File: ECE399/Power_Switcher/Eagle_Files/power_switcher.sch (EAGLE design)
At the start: 69 parts, among them J1 BANNANA_DEV, J2 BANNANA_DEV, J3 BANNANA_DEV, J4 BANNANA_DEV, J5 BANNANA_DEV, J6 BANNANA_DEV, J7 BANNANA_DEV, Q1 TRANSISTOR_DEV, Q2 TRANSISTOR_DEV, Q3 TRANSISTOR_DEV, Q4 TRANSISTOR_DEV, U1 DC_DC_DEV, U2 DC_DC_DEV, U3 GATE_DRIVER_DEV, U4 GATE_DRIVER_DEV, U5 PWM_DRIVER_DEV

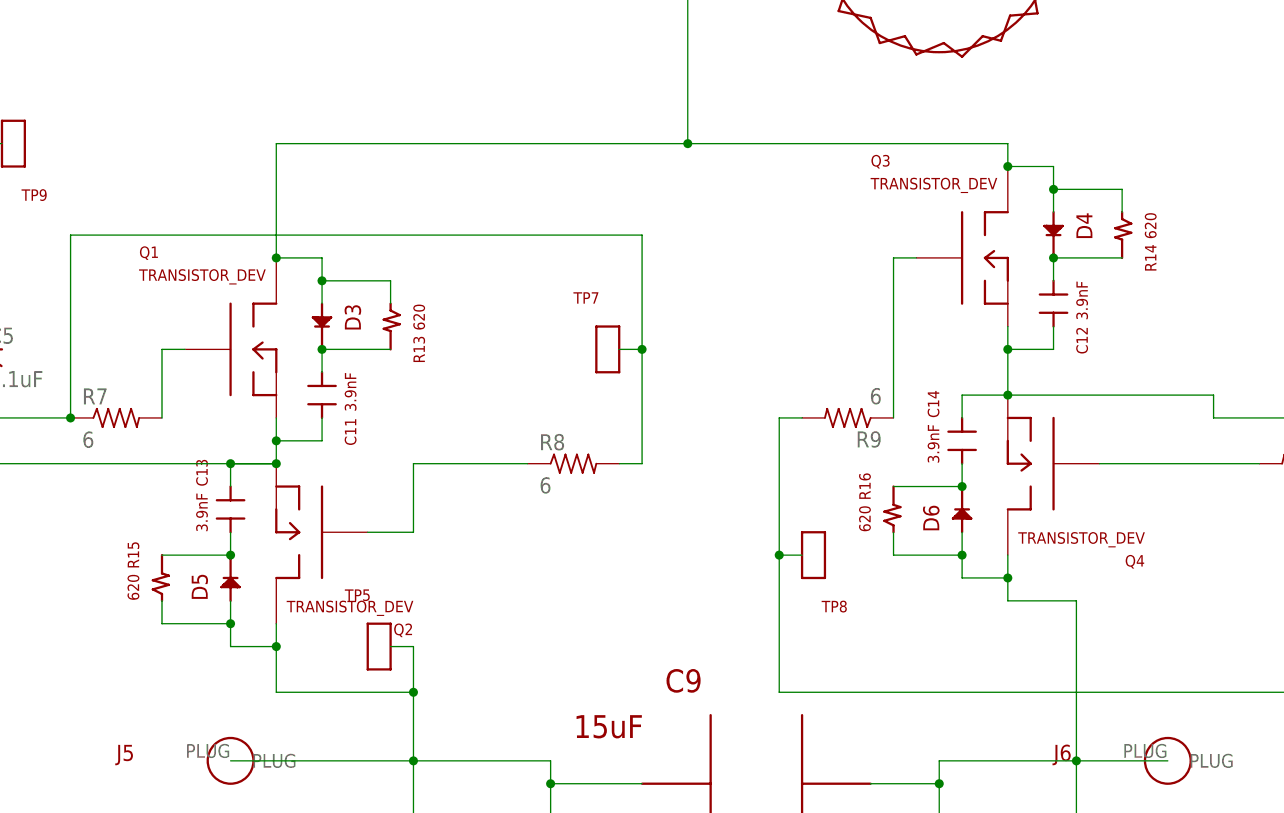
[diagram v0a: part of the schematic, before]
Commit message: right diode added
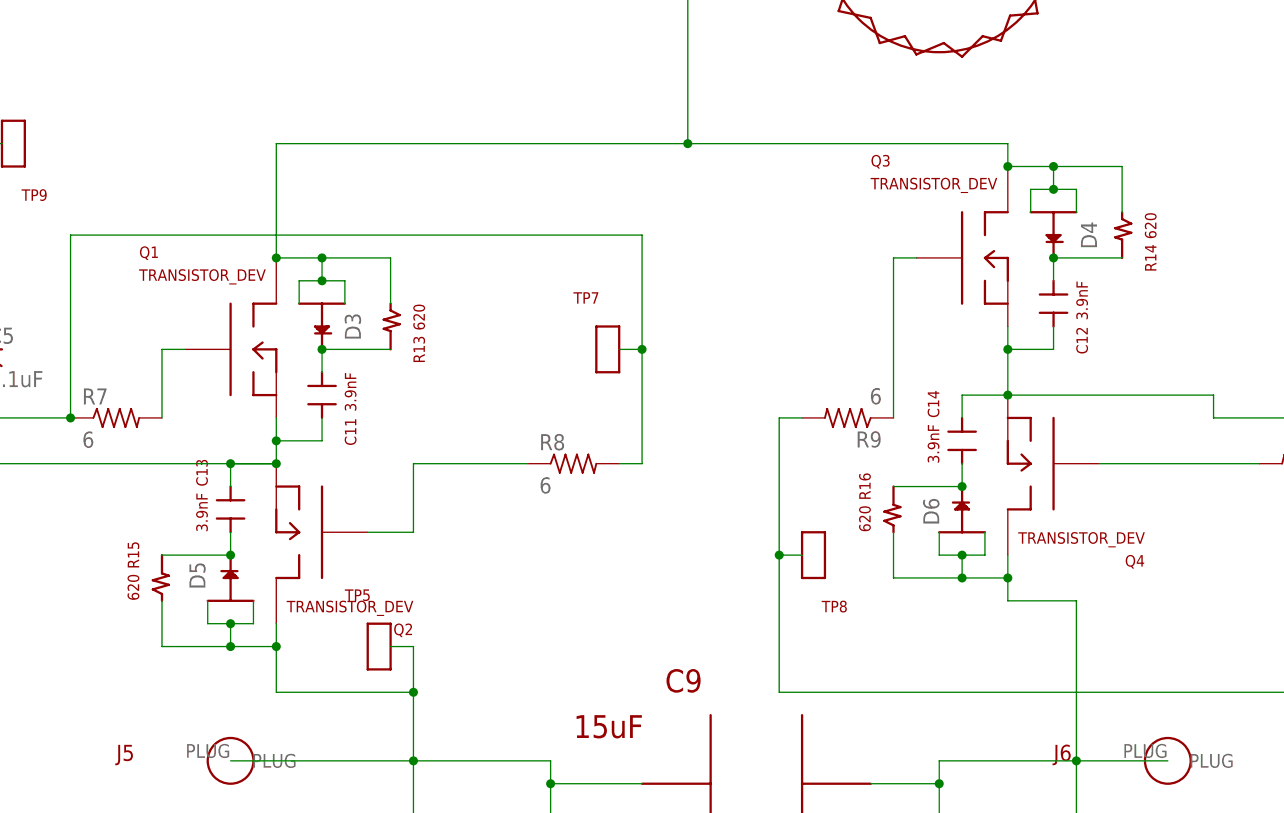
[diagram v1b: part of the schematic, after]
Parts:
- D3, D4, D5, D6: value SOD_DIODE_DEV -> D2PAK_DIODE_DEV; device power_switcher:SOD_DIODE_DEV -> blizzard_common_1:D2PAK_DIODE_DEV
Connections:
- removed net N$28: D3.P$1, D4.P$1, L3.P$2, L4.P$2, Q1.DRAIN, Q3.DRAIN, R13.P$1, R14.P$1
- new net PRE_AC_OUT: D3.IN1, D3.IN2, D4.IN1, D4.IN2, L3.P$2, L4.P$2, Q1.DRAIN, Q3.DRAIN, R13.P$1, R14.P$1
- net AC_IN_1: now also D5.IN1, D5.IN2; no longer D5.P$1
- net AC_IN_2: now also D6.IN1, D6.IN2; no longer D6.P$1
- net N$27: now also D3.OUT; no longer D3.P$2
- net N$30: now also D4.OUT; no longer D4.P$2
- net N$33: now also D5.OUT; no longer D5.P$2
- net N$36: now also D6.OUT; no longer D6.P$2
